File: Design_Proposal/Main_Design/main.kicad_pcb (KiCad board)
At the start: 2 copper layers, 100.2 x 100.2 mm, 54 parts, among them IC1 DW01A-G, IC2 TMP102AIDRLR, J1 Conn_01x33_Female, J10 Conn_01x04_Male, J2 Conn_01x33_Female, J3 MICROXNJ, J4 TP4056, J5 Conn_01x02_Male, J6 Conn_01x02_Male, J7 Conn_01x03_Male, J8 Conn_01x05_Male, J9 Conn_01x06_Male, Q1 FS8205A, U1 AMS1117-3.3, U2 1024, U3 FT232RL-REEL, U4 M24C16-RMN6TP

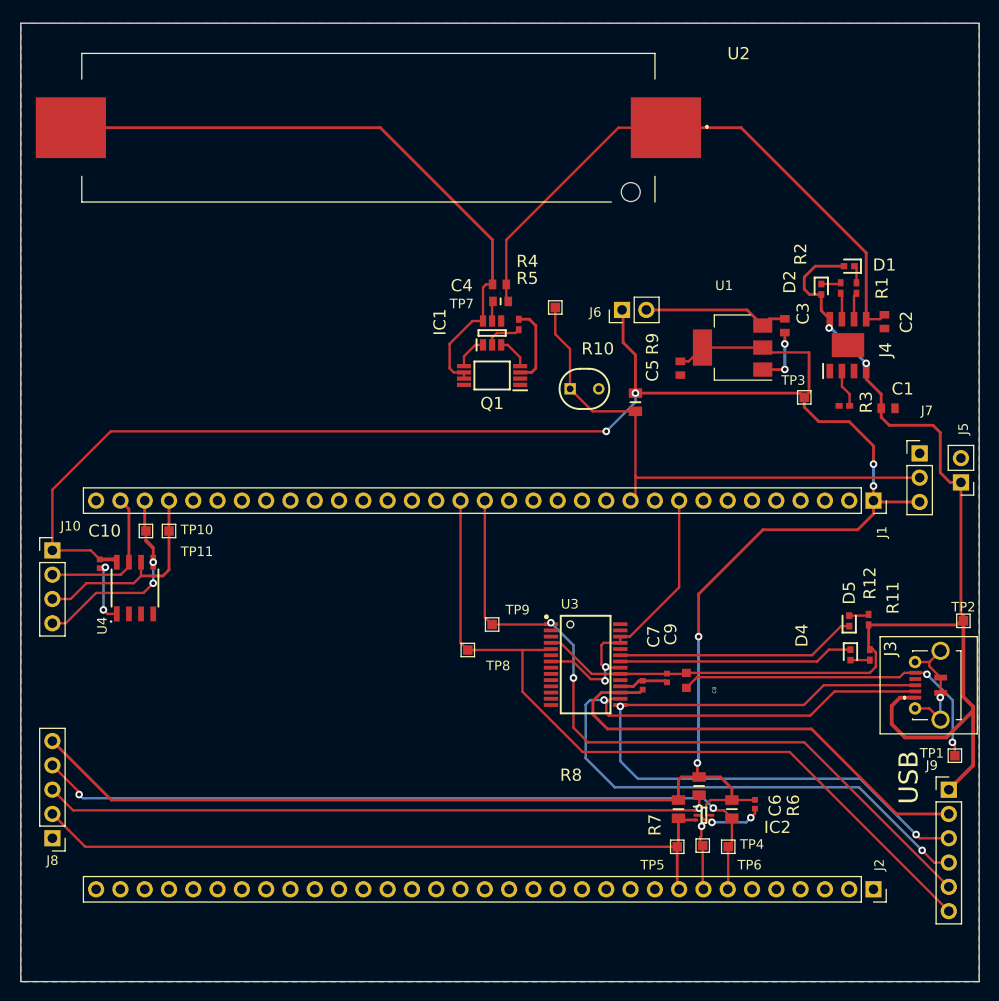
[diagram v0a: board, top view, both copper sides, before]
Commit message: update pcb
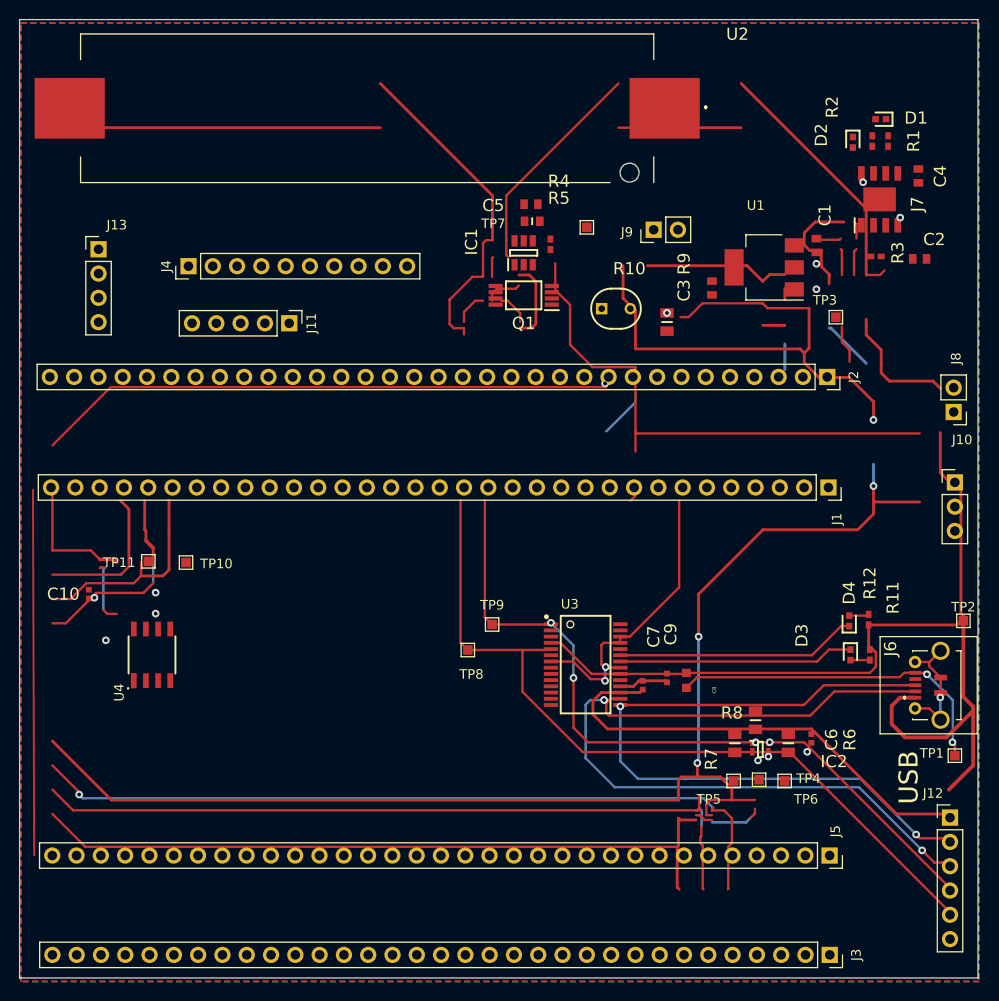
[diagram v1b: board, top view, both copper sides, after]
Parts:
- added J2: Conn_01x33_Female, Connector_PinSocket_2.54mm:PinSocket_1x33_P2.54mm_Vertical, F.Cu at (168.0, 89.3)
- added J3: Conn_01x33_Female, Connector_PinSocket_2.54mm:PinSocket_1x33_P2.54mm_Vertical, F.Cu at (168.3, 149.7)
- added J4: Conn_01x10_Female, Connector_PinHeader_2.54mm:PinHeader_1x10_P2.54mm_Vertical, F.Cu at (101.2, 77.7)
- moved J11 59.3 mm to (111.8, 83.7), turned to -90 degrees
- moved J13 31.9 mm to (91.8, 76.0)
- moved C2 16.0 mm to (177.7, 77.0)
- moved R3 16.0 mm to (173.1, 76.7)
- moved D1 15.7 mm to (173.6, 62.4)
- moved R1 15.7 mm to (174.4, 64.6)
- moved D2 15.7 mm to (170.7, 64.8)
- moved R2 15.7 mm to (172.7, 64.6)
- moved C4 15.6 mm to (177.5, 68.3)
- moved J7 15.6 mm to (173.5, 70.7)
- moved C6 9.06 mm to (166.3, 127.1)
- moved TP4 9.06 mm to (163.6, 131.5)
- moved R6 9.06 mm to (163.9, 127.6)
- moved R7 9.06 mm to (158.3, 127.6)
- moved R8 9.06 mm to (160.5, 125.2)
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- renumbered C3 to C1, C1 to C2, C5 to C3, C2 to C4, C4 to C5, D4 to D3, D5 to D4, J7 to J10, J8 to J11, J9 to J12, J10 to J13, J2 to J5, J3 to J6, J4 to J7, J5 to J8, J6 to J9
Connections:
- net 3V3 renamed /microcontroller_interfacing/3V3
- C1 pad 1: /Power/VI -> /Power/V_IN
- C2 pad 2: VCC -> +5V
- C4 pad 2: Net-(C2-Pad2) -> /Power/V_IN
- C5 pad 1: Net-(C2-Pad2) -> /Power/V_IN
- C8 pad 1: VCC -> +5V
- C9 pad 1: VCC -> +5V
- D1 pad 2: VCC -> +5V
- D2 pad 2: VCC -> +5V
- J12 pad 1: VCC -> +5V
- J6 pad 1: VCC -> +5V
- J7 pad 4: VCC -> +5V
- J7 pad 5: Net-(C2-Pad2) -> /Power/V_IN
- J7 pad 8: VCC -> +5V
- J8 pad 1: VCC -> /Power/VCC
- J9 pad 2: /Power/VI -> /Power/V_IN
- R11 pad 1: VCC -> +5V
- R12 pad 1: VCC -> +5V
- R5 pad 2: Net-(C2-Pad2) -> /Power/V_IN
- TP2 pad 1: VCC -> +5V
- U1 pad 3: /Power/VI -> /Power/V_IN
- U2 pad 1: Net-(C2-Pad2) -> /Power/V_IN
- U3 pad 20: VCC -> +5V
- U3 pad 4: VCC -> +5V
- U4 pad 1: GND -> unconnected-(U4-Pad1)
- U4 pad 2: GND -> unconnected-(U4-Pad2)
- U4 pad 3: GND -> unconnected-(U4-Pad3)
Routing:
- net GND: track 102.1 -> 329.1 mm, vias 10 -> 11
- net VCC: track 136.0 -> 0.00 mm, vias 2 -> 0
- net +5V: track 0.00 -> 127.5 mm, vias 0 -> 2
- net V_out: track 273.0 -> 150.9 mm, vias 6 -> 4
- net Alert: track 76.2 -> 0.00 mm
- net Net-(C2-Pad2): track 63.5 -> 0.00 mm
- net /NRST: track 0.00 -> 60.4 mm, vias 0 -> 1
- net ADC1: track 56.3 -> 5.26 mm
- net /Power/V_IN: track 0.00 -> 38.0 mm
- net unconnected-(J7-Pad9): track 0.00 -> 27.5 mm
- net SCL2: track 22.1 -> 0.00 mm
- net /PC4: track 0.00 -> 22.1 mm
- net Write1: track 15.6 -> 0.00 mm
- net /PB0: track 0.00 -> 15.6 mm
- net /Power/VI: track 15.3 -> 0.00 mm
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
